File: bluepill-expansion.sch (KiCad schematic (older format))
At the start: 37 parts, among them J1 SENSE_A, J10 ENCODERS, J11 LS2, J12 I/O 3V3, J13 DIGITAL_PWR, J2 SENSE_B, J3 POWER_DC, J4 MOTDC1, J5 MOTDC2, J6 I2C, J7 UART, J8 CAN_BUS, J9 LS1, SW1 LS1, SW2 LS2, U1 BluePill_STM32F103C, U2 L298HN, U3 MCP2551-I-P

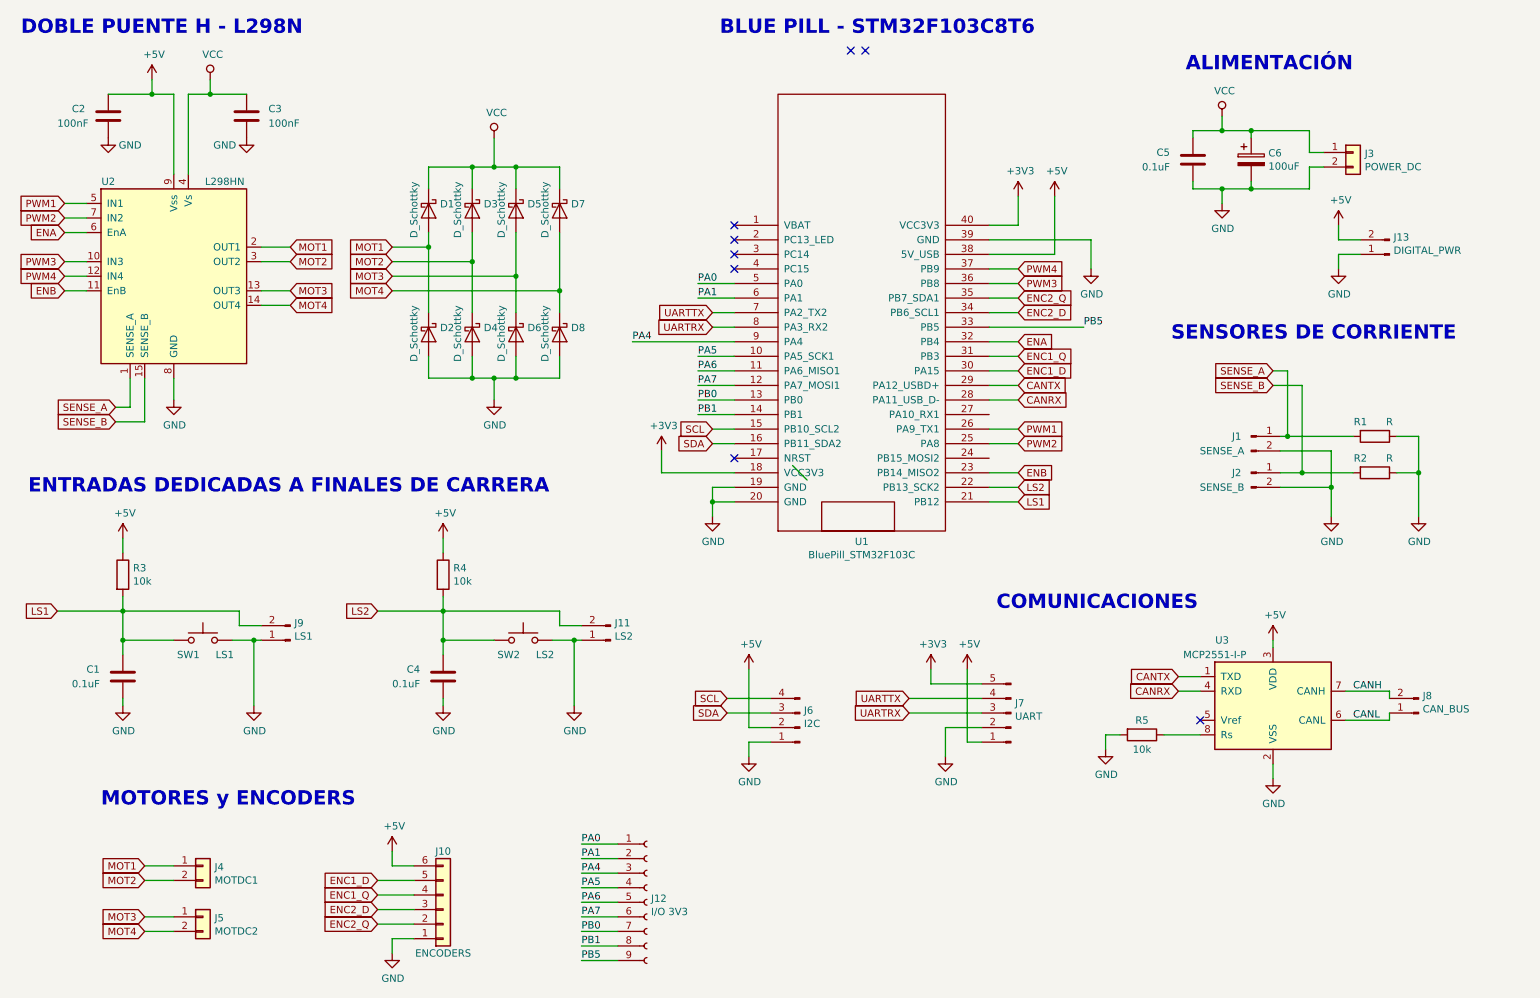
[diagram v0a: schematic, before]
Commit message: update PCB
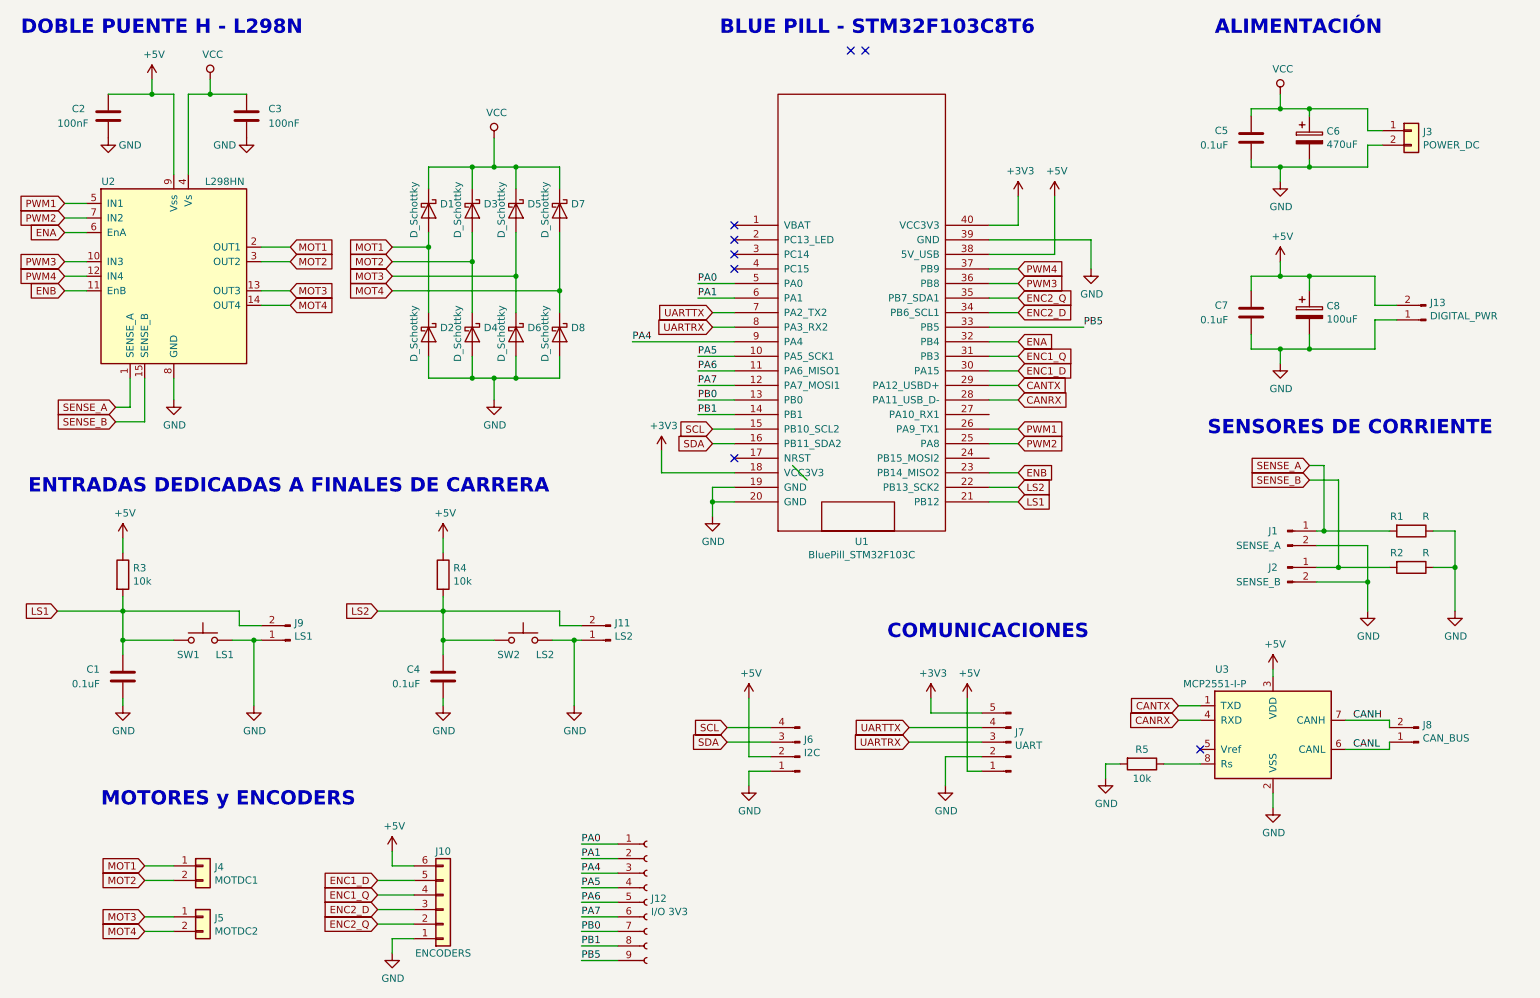
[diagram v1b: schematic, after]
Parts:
- added C7: 0.1uF, Capacitor_THT:C_Disc_D7.5mm_W2.5mm_P5.00mm, symbol Device:C
- added C8: 100uF, Capacitor_THT:CP_Radial_D5.0mm_P2.50mm, symbol Device:CP
- C6: value 100uF -> 470uF
- J13: footprint Connector_PinHeader_2.54mm:PinHeader_1x02_P2.54mm_Vertical -> TerminalBlock:TerminalBlock_bornier-2_P5.08mm
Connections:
- net +5V: now also C7.1, C8.1
- net GND: now also C7.2, C8.2
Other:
- moved on the sheet: C5, C6, J1, J13, J2, J3, J6, J7, J8, R1, R2, R5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

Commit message: 3d fixed
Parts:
- J10: footprint TerminalBlock:TerminalBlock_bornier-6_P5.08mm -> miTerminalBlock:TerminalBlock_bornier-6_P5.08mm
- J13, J3, J4, J5: footprint TerminalBlock:TerminalBlock_bornier-2_P5.08mm -> miTerminalBlock:TerminalBlock_bornier-2_P5.08mm
- SW1, SW2: footprint Button_Switch_THT:SW_PUSH_6mm_H8.5mm -> Button_Switch_THT:SW_PUSH_6mm_H7.3mm
- U2: footprint Package_TO_SOT_THT:TO-220-15_P2.54x2.54mm_StaggerOdd_Lead4.58mm_Vertical -> miPackage_TO_SOT_THT:TO-220-15_P2.54x2.54mm_StaggerOdd_Lead4.58mm_Vertical
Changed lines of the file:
@@
 F 0 "U2" H 1450 3300 50  0000 C CNN
 F 1 "L298HN" H 2250 3300 50  0000 C CNN
-F 2 "Package_TO_SOT_THT:TO-220-15_P2.54x2.54mm_StaggerOdd_Lead4.58mm_Vertical" H 1950 2000 50  0001 L CNN
+F 2 "miPackage_TO_SOT_THT:TO-220-15_P2.54x2.54mm_StaggerOdd_Lead4.58mm_Vertical" H 1950 2000 50  0001 L CNN
 F 3 "http://www.st.com/st-web-ui/static/active/en/resource/technical/document/datasheet/CD00000240.pdf" H 2050 2900 50  0001 C CNN
 	1    1900 2650
@@
 F 0 "J3" H 10480 1642 50  0000 L CNN
 F 1 "POWER_DC" H 10480 1551 50  0000 L CNN
-F 2 "TerminalBlock:TerminalBlock_bornier-2_P5.08mm" H 10400 1650 50  0001 C CNN
+F 2 "miTerminalBlock:TerminalBlock_bornier-2_P5.08mm" H 10400 1650 50  0001 C CNN
 F 3 "~" H 10400 1650 50  0001 C CNN
 	1    10400 1650
@@
 F 0 "J4" H 2180 6692 50  0000 L CNN
 F 1 "MOTDC1" H 2180 6601 50  0000 L CNN
-F 2 "TerminalBlock:TerminalBlock_bornier-2_P5.08mm" H 2100 6700 50  0001 C CNN
+F 2 "miTerminalBlock:TerminalBlock_bornier-2_P5.08mm" H 2100 6700 50  0001 C CNN
 F 3 "~" H 2100 6700 50  0001 C CNN
 	1    2100 6700
@@
 F 0 "J5" H 2180 7042 50  0000 L CNN
 F 1 "MOTDC2" H 2180 6951 50  0000 L CNN
-F 2 "TerminalBlock:TerminalBlock_bornier-2_P5.08mm" H 2100 7050 50  0001 C CNN
+F 2 "miTerminalBlock:TerminalBlock_bornier-2_P5.08mm" H 2100 7050 50  0001 C CNN
 F 3 "~" H 2100 7050 50  0001 C CNN
 	1    2100 7050
@@
 F 0 "J10" H 3750 6600 50  0000 C CNN
 F 1 "ENCODERS" H 3750 7300 50  0000 C CNN
-F 2 "TerminalBlock:TerminalBlock_bornier-6_P5.08mm" H 3750 7000 50  0001 C CNN
+F 2 "miTerminalBlock:TerminalBlock_bornier-6_P5.08mm" H 3750 7000 50  0001 C CNN
 F 3 "~" H 3750 7000 50  0001 C CNN
 	1    3750 7000
@@
 F 0 "J13" H 10472 2832 50  0000 R CNN
 F 1 "DIGITAL_PWR" H 10472 2923 50  0000 R CNN
-F 2 "TerminalBlock:TerminalBlock_bornier-2_P5.08mm" H 10500 2950 50  0001 C CNN
+F 2 "miTerminalBlock:TerminalBlock_bornier-2_P5.08mm" H 10500 2950 50  0001 C CNN
 F 3 "~" H 10500 2950 50  0001 C CNN
 	1    10500 2950
@@
 F 0 "SW1" H 2000 5050 50  0000 C CNN
 F 1 "LS1" H 2250 5050 50  0000 C CNN
-F 2 "Button_Switch_THT:SW_PUSH_6mm_H8.5mm" H 2100 5350 50  0001 C CNN
+F 2 "Button_Switch_THT:SW_PUSH_6mm_H7.3mm" H 2100 5350 50  0001 C CNN
 F 3 "~" H 2100 5350 50  0001 C CNN
 	1    2100 5150
@@
 F 0 "SW2" H 4200 5050 50  0000 C CNN
 F 1 "LS2" H 4450 5050 50  0000 C CNN
-F 2 "Button_Switch_THT:SW_PUSH_6mm_H8.5mm" H 4300 5350 50  0001 C CNN
+F 2 "Button_Switch_THT:SW_PUSH_6mm_H7.3mm" H 4300 5350 50  0001 C CNN
 F 3 "~" H 4300 5350 50  0001 C CNN
 	1    4300 5150
